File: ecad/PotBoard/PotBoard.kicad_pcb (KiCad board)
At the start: 2 copper layers, 32.7 x 35.3 mm, 6 parts, among them J1 DrivePot, J2 TonePot, J3 VolumePot

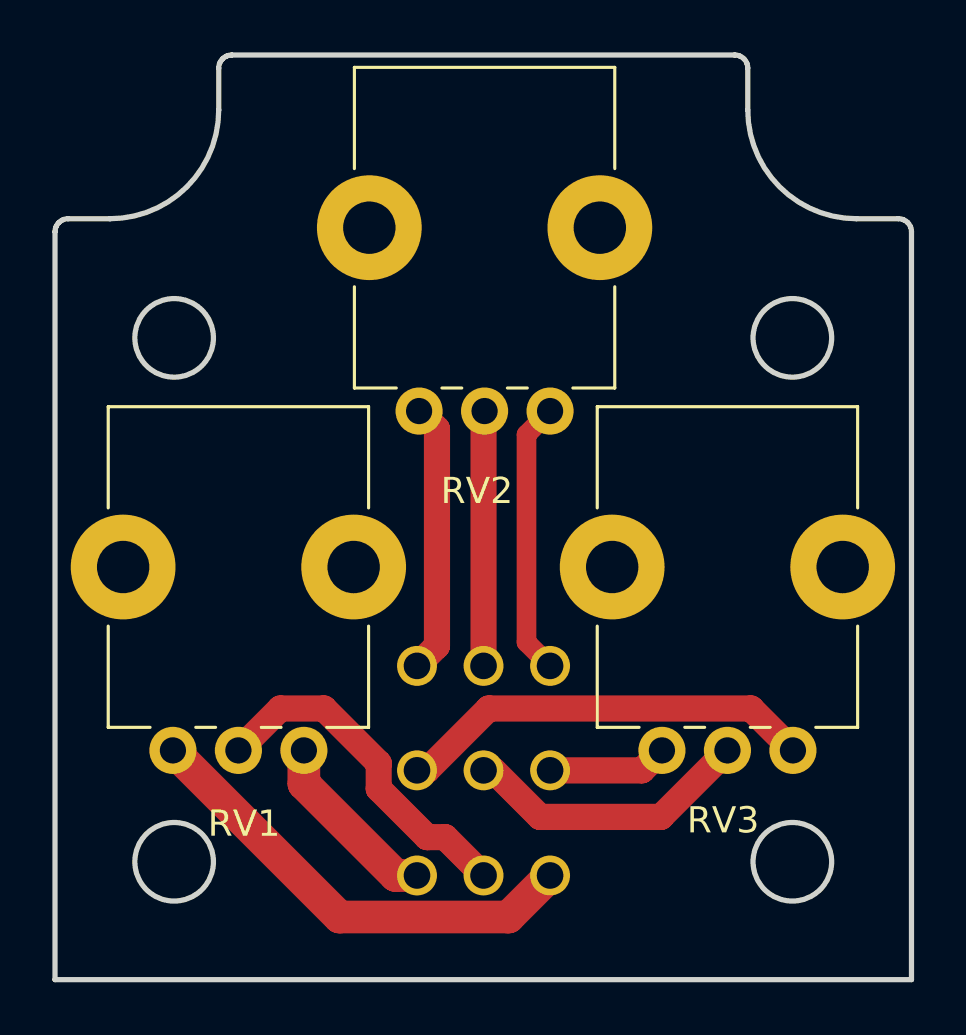
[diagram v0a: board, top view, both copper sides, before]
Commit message: Board 1v0
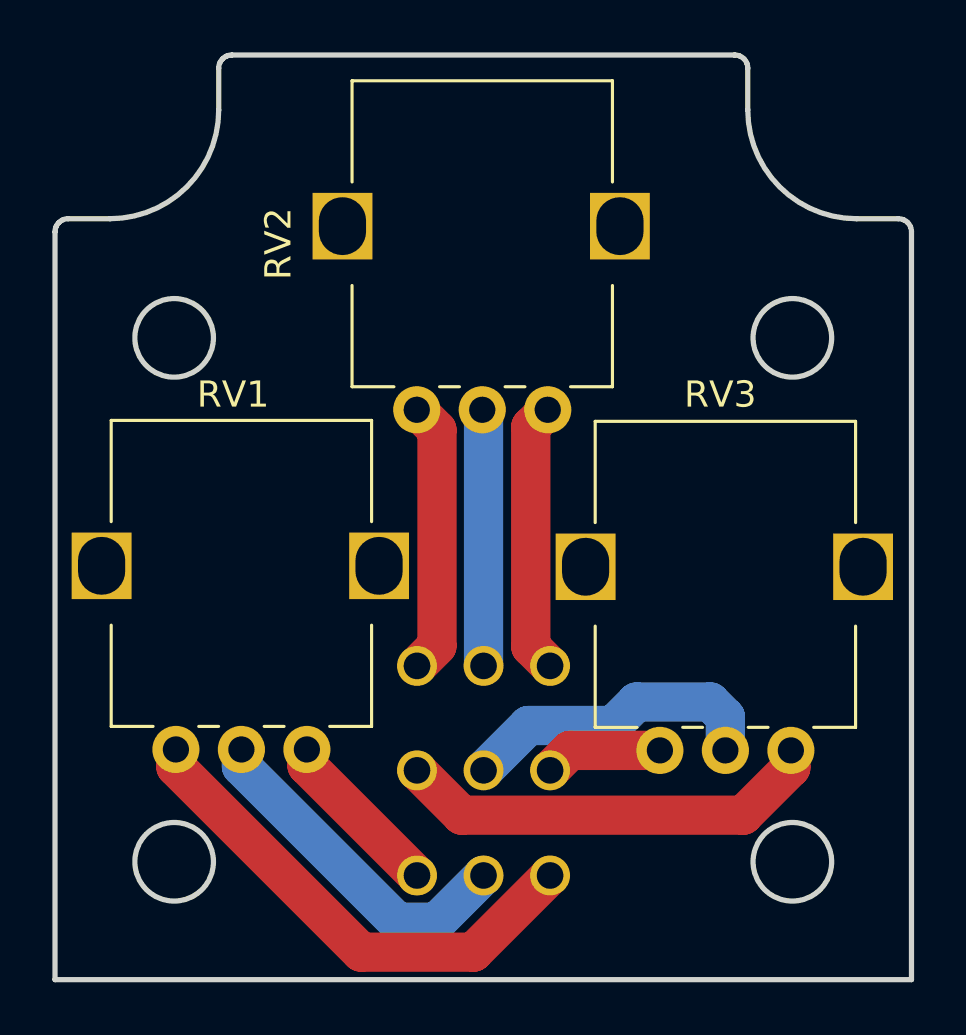
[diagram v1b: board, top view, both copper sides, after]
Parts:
- added G***: LOGO, screaming-panda:Panda_Logo, B.Cu at (130.1, 106.2)
- moved RV2 2.63 mm to (137.3, 108.7), turned to 0 degrees
- moved RV3 2.62 mm to (146.6, 121.7), turned to 0 degrees
- moved RV1 2.43 mm to (128.1, 121.6), turned to 0 degrees
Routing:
- net Net-(J1-Pad3): track 17.7 -> 19.1 mm
- net Net-(J3-Pad2): track 11.1 -> 11.8 mm
- net Net-(J2-Pad1): track 11.1 -> 10.3 mm
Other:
- board text added: "08/2022"
- board text added: "Screaming Panda 1v0"
- board text removed: "Screaming Panda 1v0 8/22"
